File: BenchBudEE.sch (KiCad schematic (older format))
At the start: 0 parts

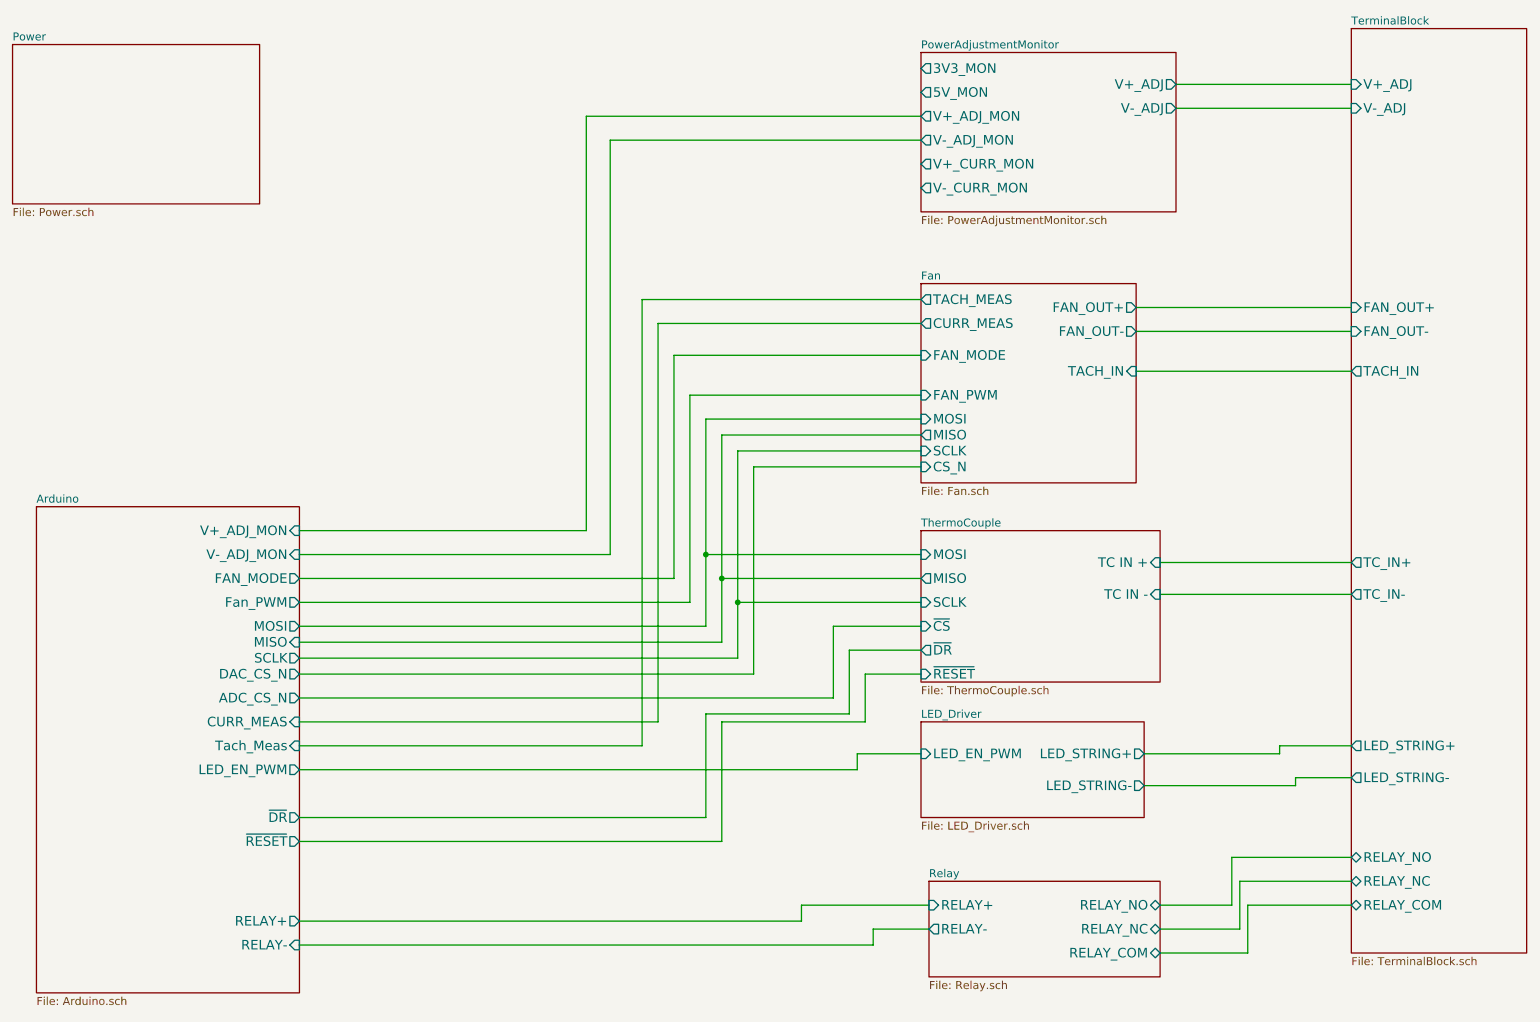
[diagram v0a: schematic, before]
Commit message: more changes?
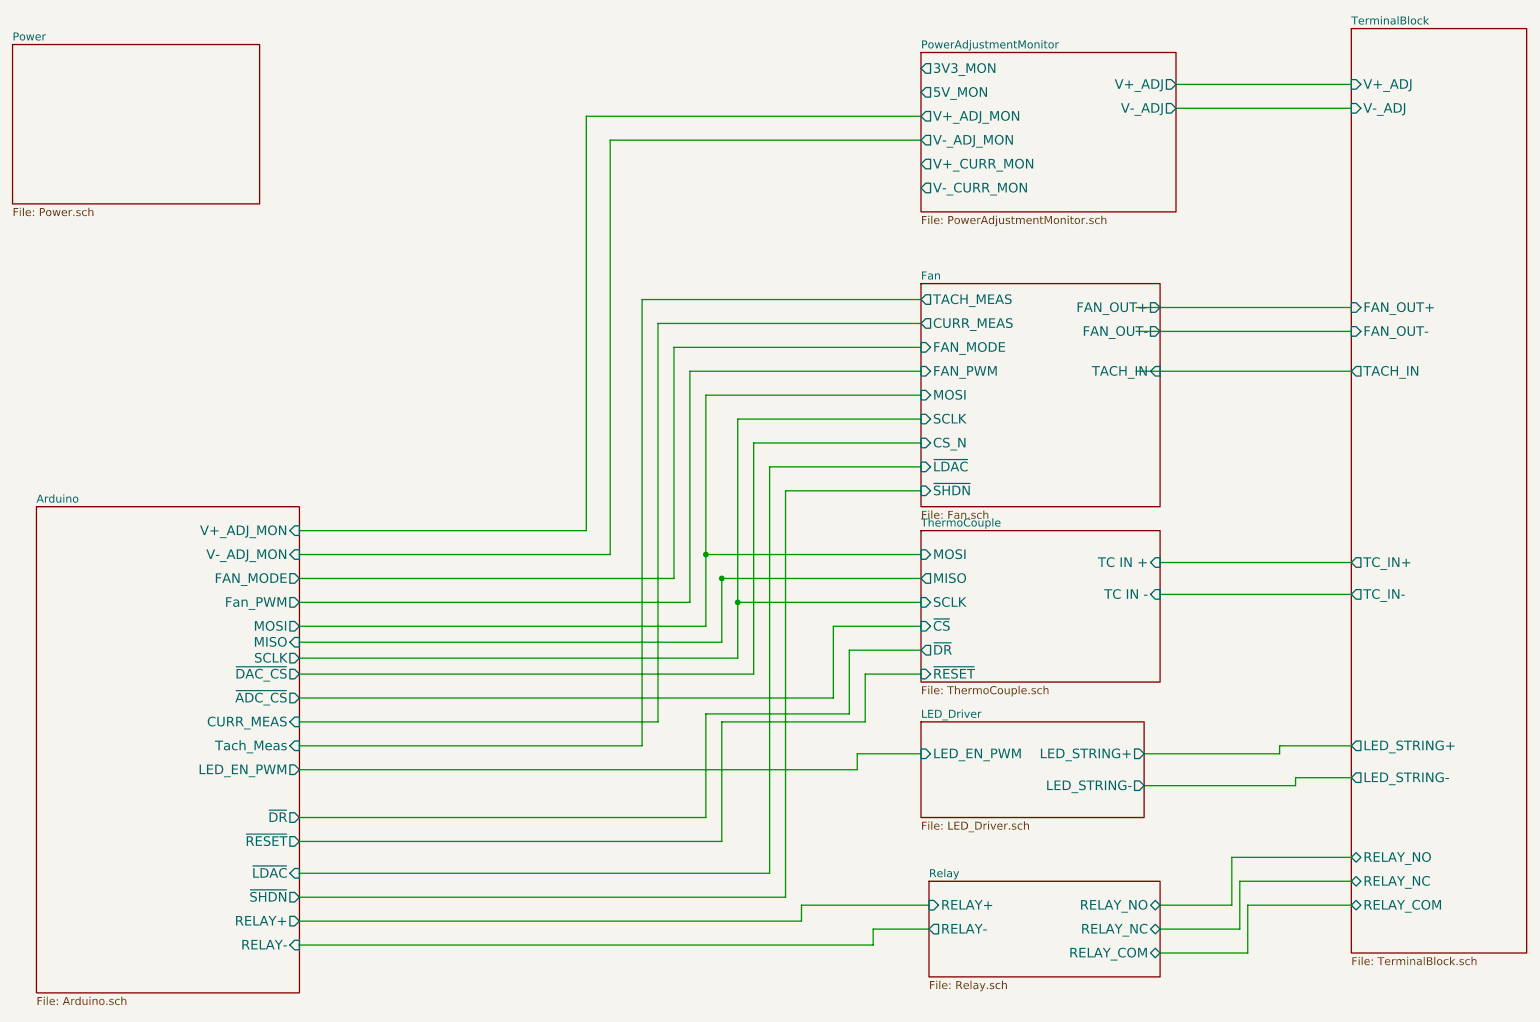
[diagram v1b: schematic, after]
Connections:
- wire segments 77 -> 82
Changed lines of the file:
@@
 $EndSheet
 $Sheet
-S 7250 2700 1350 1250
+S 7250 2700 1500 1400
 U 52ED1BE8
 F0 "Fan" 50
 F1 "Fan.sch" 50
-F2 "MOSI" I L 7250 3550 60
-F3 "MISO" O L 7250 3650 60
-F4 "SCLK" I L 7250 3750 60
-F5 "CS_N" I L 7250 3850 60
-F6 "FAN_OUT+" O R 8600 2850 60
-F7 "TACH_IN" I R 8600 3250 60
-F8 "TACH_MEAS" O L 7250 2800 60
-F9 "CURR_MEAS" O L 7250 2950 60
-F10 "FAN_OUT-" O R 8600 3000 60
-F11 "FAN_PWM" I L 7250 3400 60
-F12 "FAN_MODE" I L 7250 3150 60
+F2 "MOSI" I L 7250 3400 60
+F3 "SCLK" I L 7250 3550 60
+F4 "CS_N" I L 7250 3700 60
+F5 "FAN_OUT+" O R 8750 2850 60
+F6 "TACH_IN" I R 8750 3250 60
+F7 "TACH_MEAS" O L 7250 2800 60
+F8 "CURR_MEAS" O L 7250 2950 60
+F9 "FAN_OUT-" O R 8750 3000 60
+F10 "FAN_PWM" I L 7250 3250 60
+F11 "FAN_MODE" I L 7250 3100 60
+F12 "~LDAC" I L 7250 3850 60
+F13 "~SHDN" I L 7250 4000 60
 $EndSheet
 $Sheet
@@
 	5300 1800 7250 1800
 Wire Wire Line
-	5800 3400 7250 3400
-Wire Wire Line
-	5800 3400 5800 4700
+	5800 3250 7250 3250
+Wire Wire Line
+	5800 3250 5800 4700
 Wire Wire Line
 	5800 4700 3350 4700
@@
 F10 "V+_ADJ_MON" I R 3350 4250 60
 F11 "V-_ADJ_MON" I R 3350 4400 60
-F12 "DAC_CS_N" O R 3350 5150 60
-F13 "ADC_CS_N" O R 3350 5300 60
-F14 "Fan_PWM" O R 3350 4700 60
-F15 "FAN_MODE" O R 3350 4550 60
-F16 "~DR" O R 3350 6050 60
-F17 "~RESET" O R 3350 6200 60
-$EndSheet
-Wire Wire Line
-	7250 3550 5900 3550
-Wire Wire Line
-	5900 3550 5900 4850
+F12 "Fan_PWM" O R 3350 4700 60
+F13 "FAN_MODE" O R 3350 4550 60
+F14 "~DR" O R 3350 6050 60
+F15 "~RESET" O R 3350 6200 60
+F16 "~LDAC" I R 3350 6400 60
+F17 "~SHDN" O R 3350 6550 60
+F18 "~ADC_CS" O R 3350 5300 60
+F19 "~DAC_CS" O R 3350 5150 60
+$EndSheet
+Wire Wire Line
+	7250 3400 5900 3400
+Wire Wire Line
+	5900 3400 5900 4850
 Wire Wire Line
 	5900 4850 3350 4850
@@
 	3350 4950 6000 4950
 Wire Wire Line
-	6000 4950 6000 3650
-Wire Wire Line
-	6000 3650 7250 3650
-Wire Wire Line
-	7250 3750 6100 3750
-Wire Wire Line
-	6100 3750 6100 5050
+	7250 3550 6100 3550
+Wire Wire Line
+	6100 3550 6100 5050
 Wire Wire Line
 	6100 5050 3350 5050
@@
 	3350 5150 6200 5150
 Wire Wire Line
-	6200 5150 6200 3850
-Wire Wire Line
-	6200 3850 7250 3850
+	6200 5150 6200 3700
+Wire Wire Line
+	6200 3700 7250 3700
 Wire Wire Line
 	7250 4850 6700 4850
@@
 	6850 5650 7250 5650
 Wire Wire Line
-	7250 3150 5700 3150
-Wire Wire Line
-	5700 3150 5700 4550
+	7250 3100 5700 3100
+Wire Wire Line
+	5700 3100 5700 4550
 Wire Wire Line
 	5700 4550 3350 4550
@@
 Wire Wire Line
 	6000 6200 3350 6200
+Wire Wire Line
+	6000 4950 6000 4550
+Wire Wire Line
+	7250 3850 6300 3850
+Wire Wire Line
+	6300 3850 6300 6400
+Wire Wire Line
+	6300 6400 3350 6400
+Wire Wire Line
+	7250 4000 6400 4000
+Wire Wire Line
+	6400 4000 6400 6550
+Wire Wire Line
+	6400 6550 3350 6550
 $EndSCHEMATC
